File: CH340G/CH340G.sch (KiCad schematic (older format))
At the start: 17 parts, among them J1 USB_B_Micro, J2 Conn_01x06, U1 CH340G, Y1 Resonator

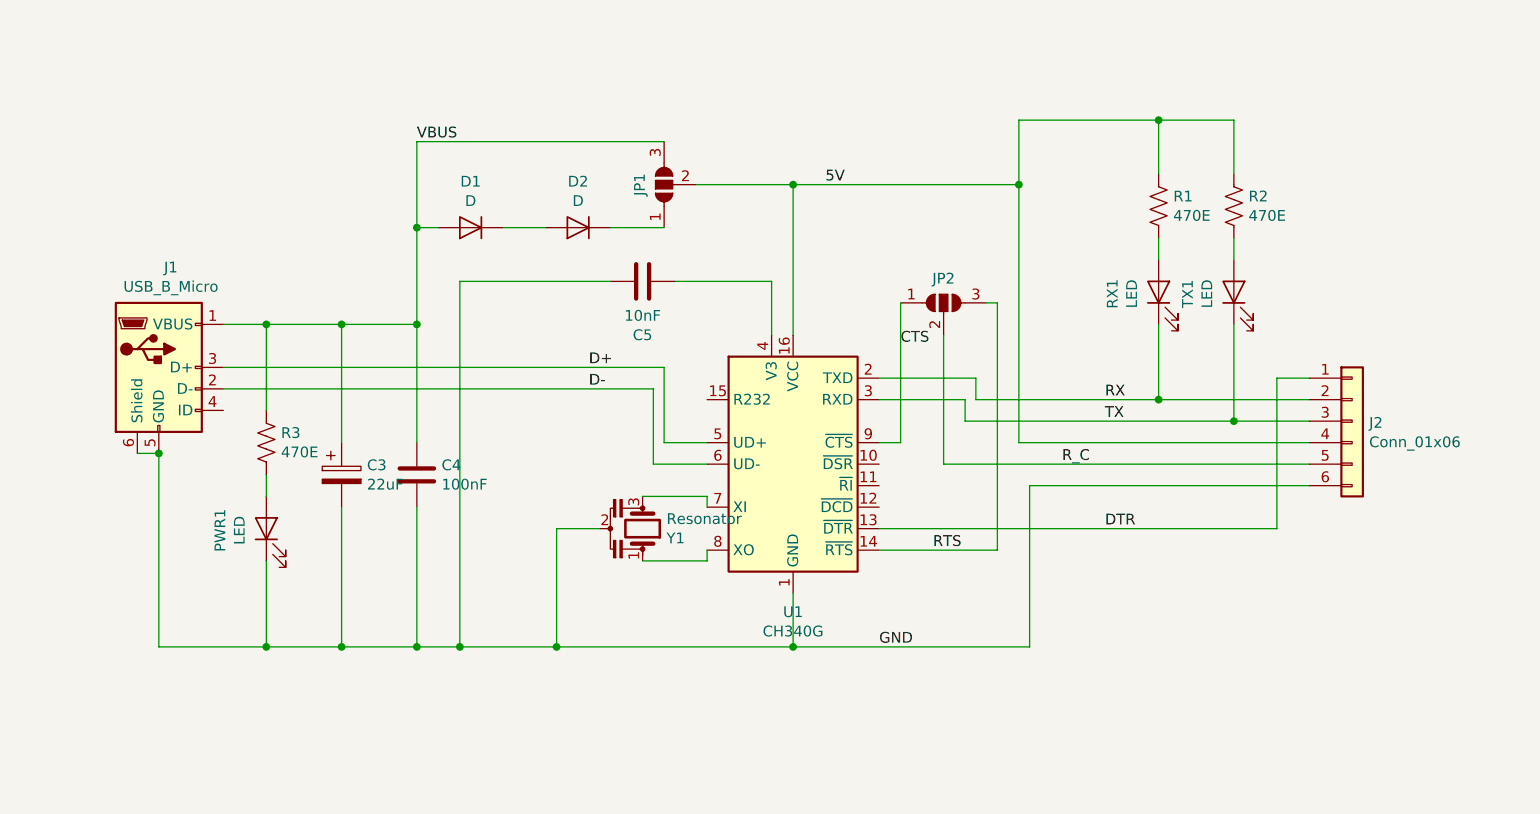
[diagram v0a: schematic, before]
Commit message: CH340G Revision 2
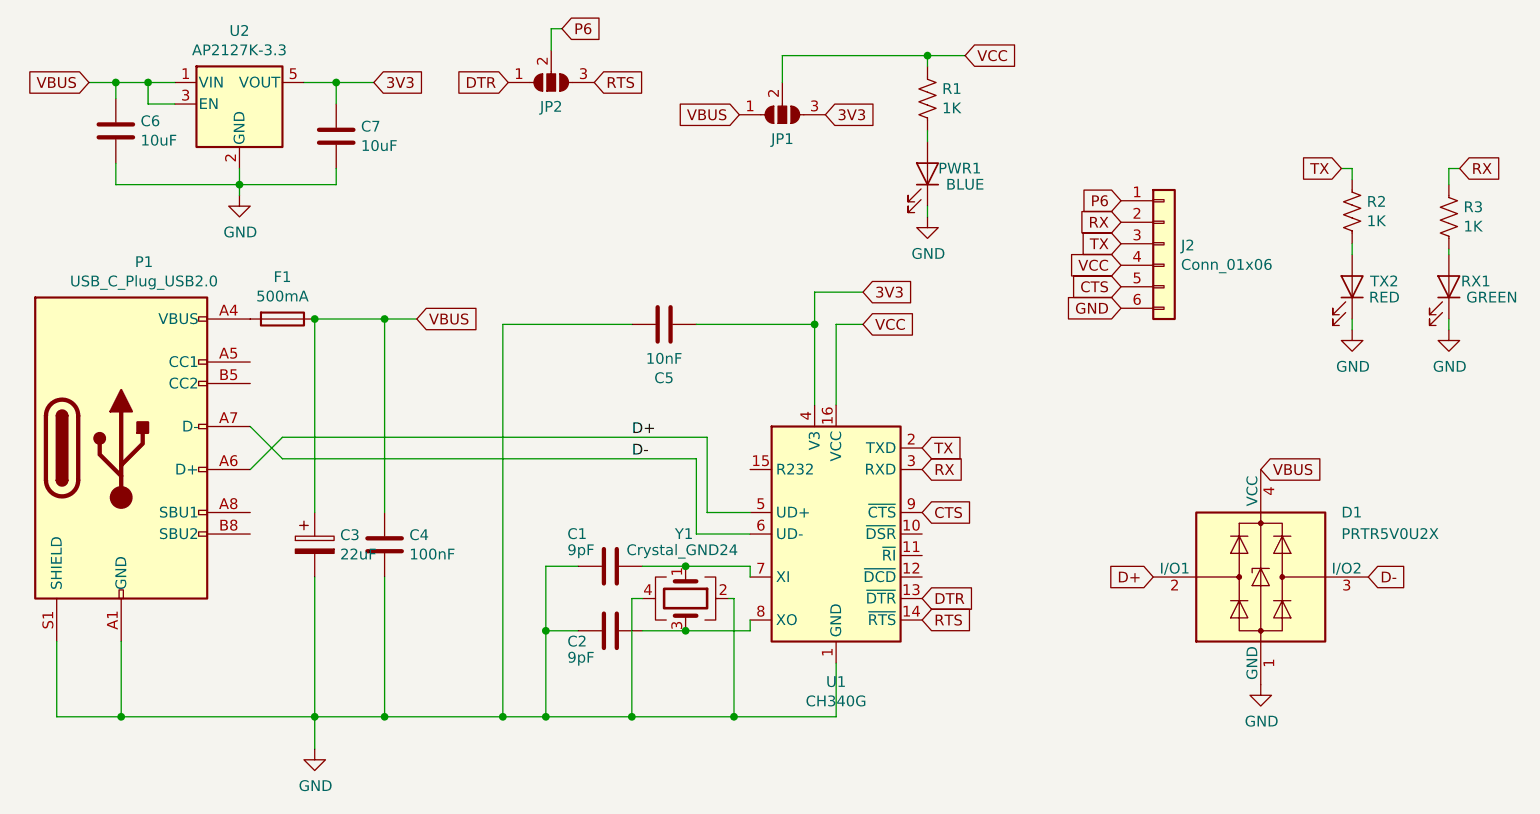
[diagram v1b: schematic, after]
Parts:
- removed D1, D2: D, Diode_SMD:D_MiniMELF, symbol Device:D
- removed J1: USB_B_Micro, Connector_USB:USB_Micro-B_Molex_47346-0001, symbol Connector:USB_B_Micro
- removed TX1: LED, LED_SMD:LED_0805_2012Metric_Castellated, symbol Device:LED
- removed Y1: Resonator, Crystal:Resonator_SMD_muRata_CSTxExxV-3Pin_3.0x1.1mm, symbol Device:Resonator
- added C1, C2: 9pF, Capacitor_SMD:C_0603_1608Metric, symbol Device:C
- added C6, C7: 10uF, Capacitor_SMD:C_0805_2012Metric, symbol Device:C
- added D1: PRTR5V0U2X, Package_TO_SOT_SMD:SOT-143, symbol Power_Protection:PRTR5V0U2X
- added F1: 500mA, Resistor_SMD:R_0805_2012Metric, symbol Device:Fuse
- added P1: USB_C_Plug_USB2.0, SirBoardLibrary:USB_C, symbol SirBoard_Library:USB_C_Plug_USB2.0
- added TX2: RED, LED_SMD:LED_0603_1608Metric, symbol Device:LED
- added U2: AP2127K-3.3, Package_TO_SOT_SMD:SOT-23-5, symbol Regulator_Linear:AP2127K-3.3
- added Y1: Crystal_GND24, Crystal:Crystal_SMD_SeikoEpson_TSX3225-4Pin_3.2x2.5mm, symbol Device:Crystal_GND24
- C3: Part (none) -> C122643
- C4: footprint Capacitor_SMD:C_0805_2012Metric_Pad1.15x1.40mm_HandSolder -> Capacitor_SMD:C_0603_1608Metric; Part (none) -> C42998
- C5: footprint Capacitor_SMD:C_0805_2012Metric_Pad1.15x1.40mm_HandSolder -> Capacitor_SMD:C_0603_1608Metric; Part (none) -> C100042
- PWR1: value LED -> BLUE; footprint LED_SMD:LED_0805_2012Metric_Castellated -> LED_SMD:LED_0603_1608Metric; Part (none) -> C193191
- R1, R2: value 470E -> 1K; footprint Resistor_SMD:R_0805_2012Metric_Pad1.15x1.40mm_HandSolder -> Resistor_SMD:R_0603_1608Metric; Part (none) -> C269441
- R3: value 470E -> 1K; footprint Resistor_SMD:R_0805_2012Metric_Pad1.15x1.40mm_HandSolder -> Resistor_SMD:R_0603_1608Metric; Part (none) -> C25585
- RX1: value LED -> GREEN; footprint LED_SMD:LED_0805_2012Metric_Castellated -> LED_SMD:LED_0603_1608Metric; Part (none) -> C205443
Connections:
- net CTS: now also J2.5 (Pin_5); no longer JP2.1 (A)
- net D+: now also D1.2 (I/O1), P1.A6 (D+), P1.B6 (D+)
- net D-: now also D1.3 (I/O2), P1.A7 (D-), P1.B7 (D-)
- net DTR: now also JP2.1 (A); no longer J2.1 (Pin_1)
- net GND: now also RX1.1 (K), C1.2, C2.2, C6.2, C7.2, D1.1 (GND), P1.A1 (GND), P1.A12 (GND), P1.B1 (GND), P1.B12 (GND), P1.S1 (SHIELD), TX2.1 (K), U2.2 (GND), Y1.2, Y1.4
- net RX: now also R3.1, U1.3 (RXD); no longer RX1.1 (K), U1.2 (TXD)
- net TX: now also R2.1, U1.2 (TXD); no longer U1.3 (RXD)
- net VBUS: now also JP1.1 (A), C6.1, D1.4 (VCC), F1.1, U2.1 (VIN), U2.3 (EN); no longer JP1.3 (B), R3.1
- net 3V3: now reaches C5.2, U1.4 (V3)
- net 3V3: now also JP1.3 (B), C7.1, U2.5 (VOUT)
- net at U1.7 (XI): now also C1.1, Y1.1
- net at U1.8 (XO): now also C2.1, Y1.3
- net at RX1.2 (A): now also R3.2; no longer R1.2
- net at R2.2: now also TX2.2 (A)
- net at PWR1.2 (A): now also R1.2; no longer R3.2
- net 5V renamed VCC
- net VCC: no longer R2.1
- net R_C renamed P6
- net P6: now also J2.1 (Pin_1); no longer J2.5 (Pin_5)
- new net: F1.2, P1.A4 (VBUS), P1.A9 (VBUS), P1.B4 (VBUS), P1.B9 (VBUS)
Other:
- moved on the sheet: C3, C4, C5, J2, JP1, JP2, U1
